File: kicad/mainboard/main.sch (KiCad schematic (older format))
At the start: 34 parts, among them IC2 LM358D, IC3 MC34063AD, J1 Power, J2 GM Tube, Q1 IRF840, Q2 Q_PNP_BEC, Q3 BC848SMD, Q4 BC848SMD

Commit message: directory structure change
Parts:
- removed J1: Power, Pin_Headers:Pin_Header_Angled_1x02_Pitch2.54mm, symbol main-eagle-import:22-?-0205-7028
- removed J2: GM Tube, Pin_Headers:Pin_Header_Angled_1x02_Pitch2.54mm, symbol main-eagle-import:22-?-0205-7028
- removed JP1: JP1E, Pin_Headers:Pin_Header_Straight_1x02_Pitch2.54mm, symbol main-eagle-import:JP1E
- removed SV2: Digital Output, Pin_Headers:Pin_Header_Straight_1x03_Pitch2.54mm, symbol main-eagle-import:MA03-1
- added C8: 330u, Capacitor_Tantalum_SMD:CP_EIA-3528-21_Kemet-B, symbol Device:CP
- added C9: 10n, Capacitor_SMD:C_0805_2012Metric_Pad1.15x1.40mm_HandSolder, symbol main-eagle-import:C-EUC0805
- added D4: D_Zener, Diode_THT:D_A-405_P2.54mm_Vertical_KathodeUp, symbol Device:D_Zener
- added J1, J2, J3: Conn_01x02_Male, Connector_PinHeader_2.54mm:PinHeader_1x02_P2.54mm_Horizontal, symbol Connector:Conn_01x02_Male
- added J4: Conn_01x03_Male, Connector_PinHeader_2.54mm:PinHeader_1x03_P2.54mm_Vertical, symbol Connector:Conn_01x03_Male
- added J5: Conn_01x02_Male, Connector_PinHeader_2.54mm:PinHeader_1x02_P2.54mm_Vertical, symbol Connector:Conn_01x02_Male
- added JP1: Jumper_3_Bridged12, Jumper:SolderJumper-3_P1.3mm_Bridged12_Pad1.0x1.5mm, symbol Jumper:Jumper_3_Bridged12
- C1, C2, C3, C4, C6: footprint Capacitors_SMD:C_0805_HandSoldering -> Capacitor_SMD:C_0805_2012Metric_Pad1.15x1.40mm_HandSolder
- C5: footprint Capacitors_THT:C_Axial_L12.0mm_D7.5mm_P15.00mm_Horizontal -> Capacitor_THT:C_Rect_L13.0mm_W6.5mm_P7.50mm_P10.00mm
- C7: footprint Capacitors_Tantalum_SMD:CP_Tantalum_Case-B_EIA-3528-21_Hand -> Capacitor_Tantalum_SMD:CP_EIA-3528-21_Kemet-B
- D2: footprint Diodes_THT:D_DO-41_SOD81_P7.62mm_Horizontal -> Diode_THT:D_DO-41_SOD81_P7.62mm_Horizontal
- D3: footprint LEDs:LED_D3.0mm -> LED_THT:LED_D3.0mm
- L1: footprint Inductors_THT:L_Radial_D7.5mm_P5.00mm_Fastron_07P -> Inductor_THT:L_Radial_D7.5mm_P5.00mm_Fastron_07P
- Q1: footprint TO_SOT_Packages_THT:TO-220-3_Vertical -> Package_TO_SOT_THT:TO-220-3_Vertical
- R1, R11, R12, R13, R14, R4, R5, R8, R9: footprint Resistors_SMD:R_0805_HandSoldering -> Resistor_SMD:R_0805_2012Metric_Pad1.15x1.40mm_HandSolder
- R2: footprint Resistors_THT:R_Axial_DIN0207_L6.3mm_D2.5mm_P2.54mm_Vertical -> Resistor_THT:R_Axial_DIN0207_L6.3mm_D2.5mm_P2.54mm_Vertical
- R3: footprint Resistors_THT:R_Axial_DIN0207_L6.3mm_D2.5mm_P5.08mm_Vertical -> Resistor_THT:R_Axial_DIN0207_L6.3mm_D2.5mm_P5.08mm_Vertical
- R6: footprint Resistors_THT:R_Axial_DIN0207_L6.3mm_D2.5mm_P5.08mm_Vertical -> Resistor_THT:R_Axial_DIN0207_L6.3mm_D2.5mm_P7.62mm_Horizontal
- R7: footprint Resistors_THT:R_Axial_DIN0207_L6.3mm_D2.5mm_P2.54mm_Vertical -> Resistor_SMD:R_0805_2012Metric_Pad1.15x1.40mm_HandSolder
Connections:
- wire segments 146 -> 168
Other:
- note added: "5V power supply"
- note removed: "Power supply"
- moved on the sheet: R13, R2

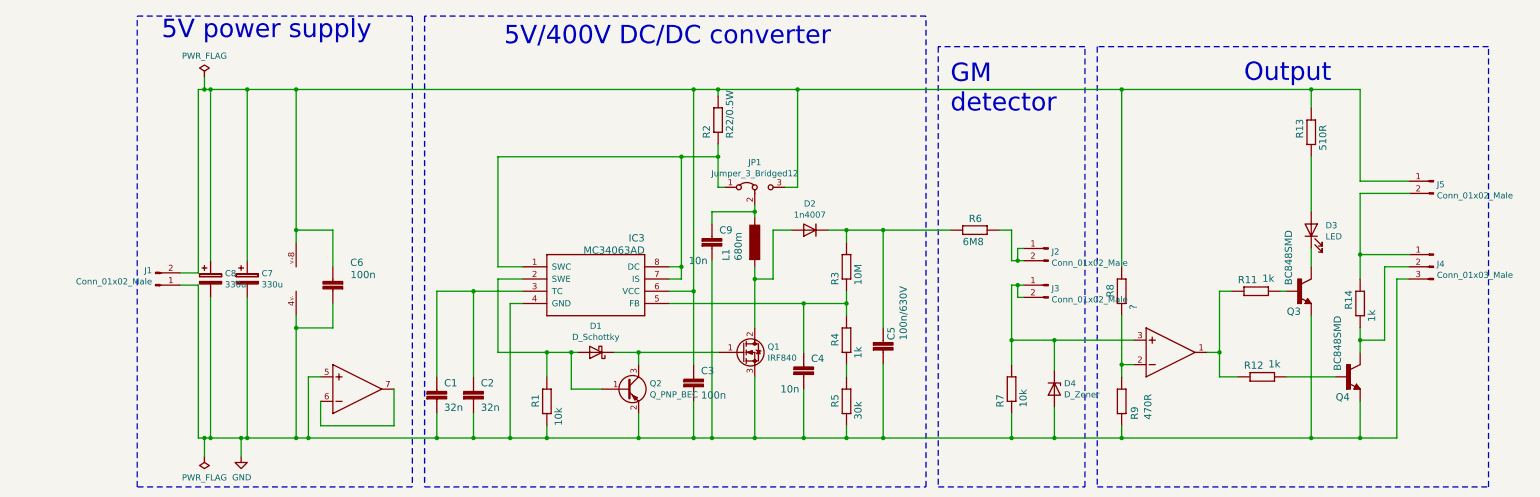
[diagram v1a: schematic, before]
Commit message: new hw ready to be send to pcb company
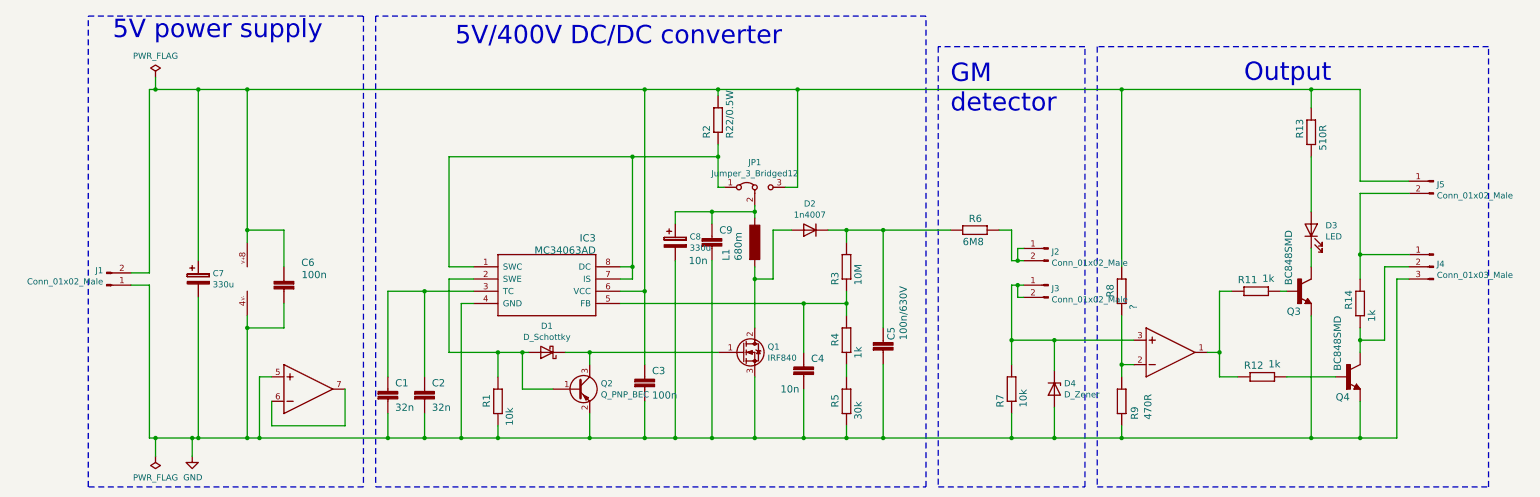
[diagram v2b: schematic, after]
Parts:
- C5: footprint Capacitor_THT:C_Rect_L13.0mm_W6.5mm_P7.50mm_P10.00mm -> Capacitors_THT:C_Rect_L13.5mm_W5.0mm_P10.00mm_FKS3_FKP3_MKS4
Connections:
- net at C3.1, C6.1, C7.1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: no longer C8.1
- net at C9.1, JP1.2 (C), L1.1: now also C8.1
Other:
- moved on the sheet: C1, C2, C3, C6, C7, C8, D1, IC3, J1, Q2, R1
